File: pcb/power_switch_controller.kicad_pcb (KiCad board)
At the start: 2 copper layers, 118.1 x 54.6 mm, 63 parts, among them P1 PWR_JACK_2.5x5.5, P2 HEADER_01X03, P3 BNC_DOUBLE_RA, P4 HEADER_02X08_SMD, P5 HEADER_02X08_SMD, P6 HEADER_02X08_SMD, P7 HEADER_02X08_SMD, SW1 DPST_SERIES_M, SW2 KT_SWITCH, U1 MAX6817, U2 MAX6817, U3 TLE723X, U4 TLE723X, U5 TLE723X, U6 TLE723X

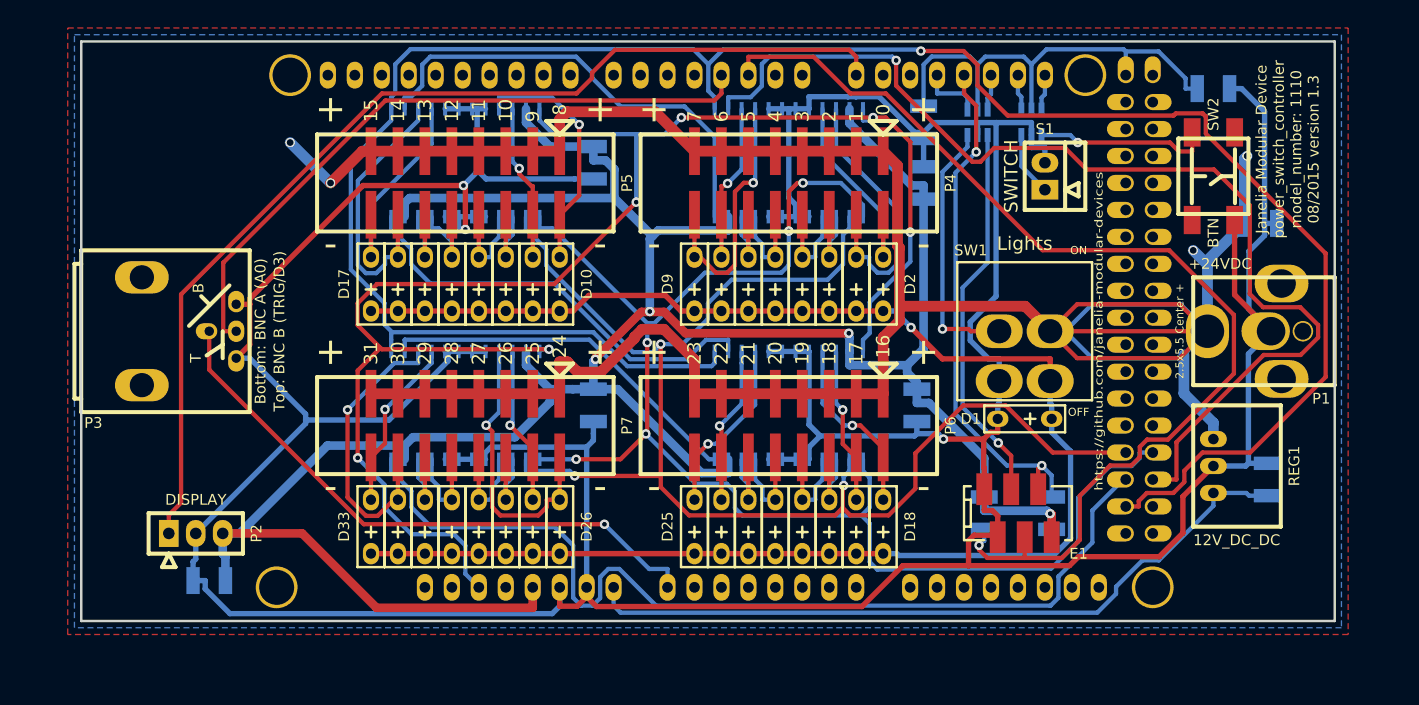
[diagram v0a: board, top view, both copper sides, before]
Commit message: Progress towards pcb v1.4.
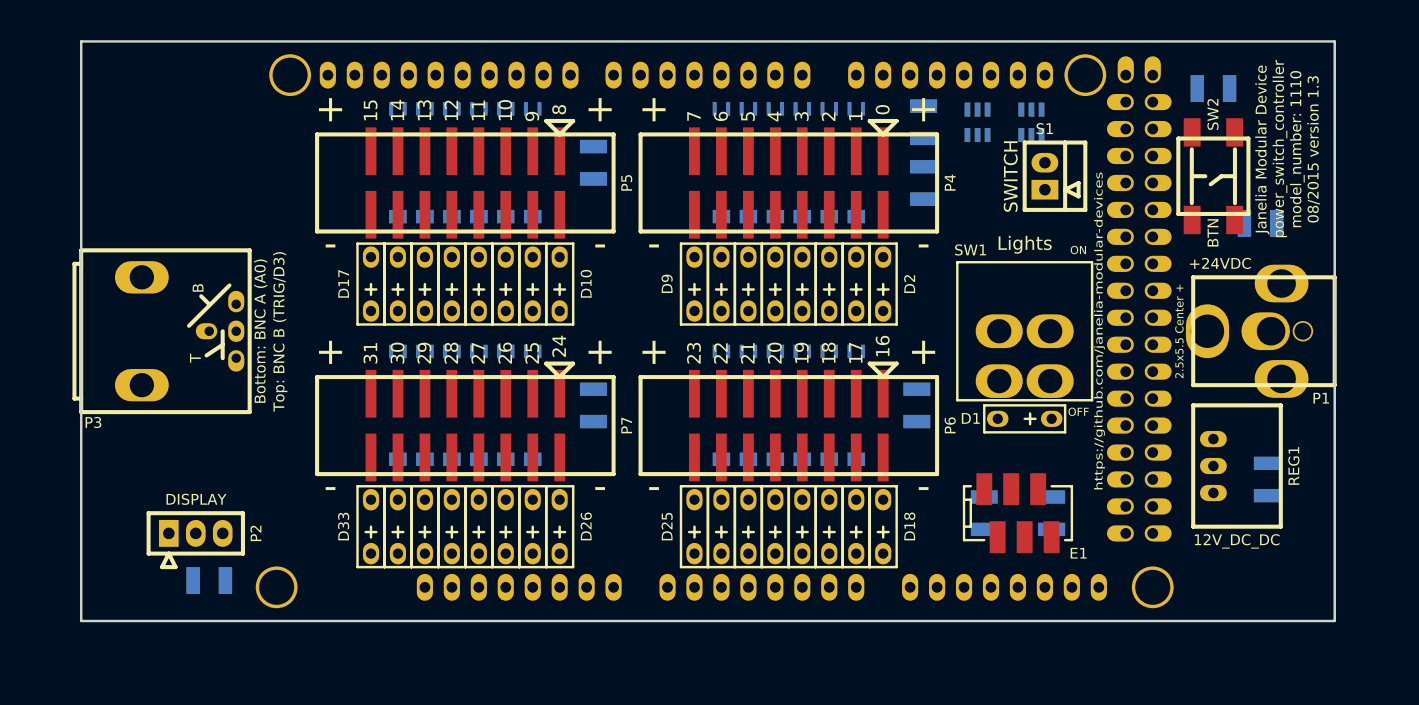
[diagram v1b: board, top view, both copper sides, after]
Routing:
- net GND: track 449.0 -> 0.00 mm, vias 3 -> 0
- net VAA: track 270.6 -> 0.00 mm, vias 4 -> 0
- net +5V: track 254.0 -> 0.00 mm, vias 4 -> 0
- net /SCK: track 203.9 -> 0.00 mm, vias 1 -> 0
- net /LED_PWR: track 151.6 -> 0.00 mm, vias 1 -> 0
- net /RST: track 151.1 -> 0.00 mm, vias 6 -> 0
- net /CS: track 137.5 -> 0.00 mm, vias 5 -> 0
- net /IN: track 131.6 -> 0.00 mm, vias 3 -> 0
- net /ENC_B: track 101.7 -> 0.00 mm, vias 1 -> 0
- net /MOSI: track 101.7 -> 0.00 mm, vias 1 -> 0
- net /TX3: track 98.5 -> 0.00 mm
- net /MISO: track 91.2 -> 0.00 mm
- net /V_IN: track 69.5 -> 0.00 mm
- net /BNC_B: track 63.0 -> 0.00 mm
- net /BNC_A: track 56.3 -> 0.00 mm, vias 1 -> 0
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- removed copper zone on B.Cu, net GND
- removed copper zone on F.Cu, net VAA

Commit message: Updated bom.
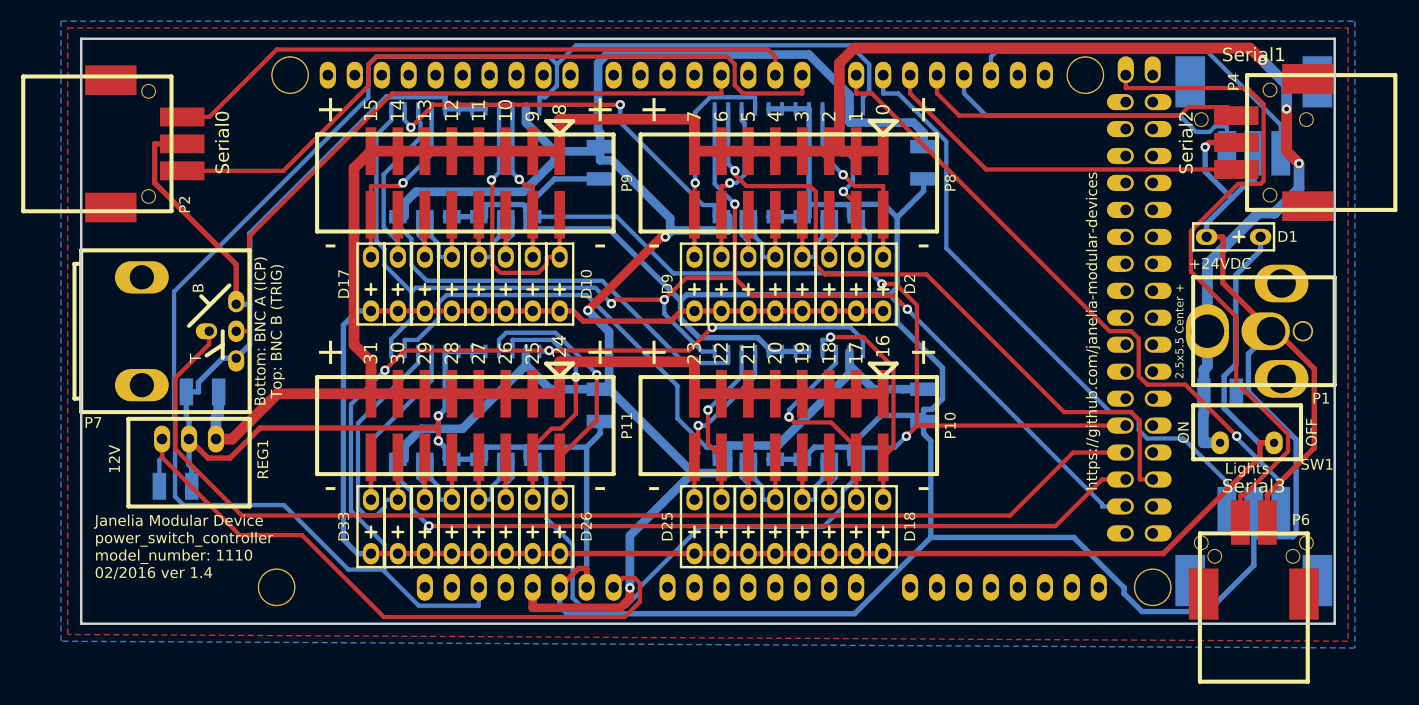
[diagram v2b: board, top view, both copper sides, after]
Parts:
- removed C8, C9: 0.1uF, power_switch_controller:SM1210
- removed E1: ENCODER_C14, power_switch_controller:Micro-MaTch_6_SMD
- removed R1, R2: 5.11k, power_switch_controller:SM1210
- removed S1: HEADER_01X02_SHR, power_switch_controller:Header_Shrouded_2_Pin
- removed SW2: KT_SWITCH, power_switch_controller:KT_SWITCH
- removed U5, U6: TLE723X, power_switch_controller:TLE723X
- added P10: HEADER_02X08_SMD, power_switch_controller:HEADER_02x08_SMD, F.Cu at (160.0, 111.8)
- added P11: HEADER_02X08_SMD, power_switch_controller:HEADER_02x08_SMD, F.Cu at (129.5, 111.8)
- added P8: HEADER_02X08_SMD, power_switch_controller:HEADER_02x08_SMD, F.Cu at (160.0, 88.9)
- added P9: HEADER_02X08_SMD, power_switch_controller:HEADER_02x08_SMD, F.Cu at (129.5, 88.9)
- P2: value HEADER_01X03 -> HEADER_01X03_SMD_RA; footprint footprints:Header_3_Pin -> power_switch_controller:Header_3_Pin_SMD_RA
- P3: value BNC_DOUBLE_RA -> HEADER_01X03_SMD_RA; footprint power_switch_controller:BNC_DOUBLE -> power_switch_controller:Header_3_Pin_SMD_RA; moved to B.Cu
- P4: value HEADER_02X08_SMD -> HEADER_01X03_SMD_RA; footprint power_switch_controller:HEADER_02x08_SMD -> power_switch_controller:Header_3_Pin_SMD_RA
- P5: value HEADER_02X08_SMD -> HEADER_01X03_SMD_RA; footprint power_switch_controller:HEADER_02x08_SMD -> power_switch_controller:Header_3_Pin_SMD_RA; moved to B.Cu
- P6: value HEADER_02X08_SMD -> HEADER_01X02_SMD_RA; footprint power_switch_controller:HEADER_02x08_SMD -> power_switch_controller:Header_2_Pin_SMD_RA
- P7: value HEADER_02X08_SMD -> BNC_DOUBLE_RA; footprint power_switch_controller:HEADER_02x08_SMD -> power_switch_controller:BNC_DOUBLE
- SW1: value DPST_SERIES_M -> SPST_SLIDE_AS; footprint power_switch_controller:DPST_SERIES_M -> power_switch_controller:SPST_SLIDE_AS
- U1, U2: value MAX6817 -> TLE723X; footprint power_switch_controller:MAX6817 -> power_switch_controller:TLE723X
- moved P3 107.4 mm to (203.8, 79.4), turned to 180 degrees
- moved C2 100.7 mm to (104.8, 108.6), turned to 180 degrees
- moved REG1 96.6 mm to (103.5, 113.0), turned to 180 degrees
- moved P5 83.2 mm to (203.8, 126.4)
- moved C5 58.2 mm to (142.2, 87.0), turned to 270 degrees
- moved U2 53.5 mm to (129.5, 87.0), turned to 180 degrees
- moved P4 49.0 mm to (208.9, 85.1), turned to 270 degrees
- moved P6 46.6 mm to (203.8, 127.6), turned to 180 degrees
- moved P2 37.6 mm to (96.1, 85.2), turned to 90 degrees
- moved P7 31.7 mm to (99.1, 102.9), turned to 90 degrees
- moved D1 26.1 mm to (201.9, 94.0)
- moved SW1 23.0 mm to (203.2, 112.4), turned to 90 degrees
- moved C7 22.9 mm to (142.2, 109.9)
- moved U3 22.9 mm to (160.0, 109.9)
- moved U4 22.9 mm to (129.5, 109.9)
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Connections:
- ARDUINO1 pad 0: Net-(ARDUINO1-Pad0) -> /RX0
- ARDUINO1 pad 1: Net-(ARDUINO1-Pad1) -> /TX0
- ARDUINO1 pad 10: Net-(ARDUINO1-Pad10) -> (no net)
- ARDUINO1 pad 11: Net-(ARDUINO1-Pad11) -> (no net)
- ARDUINO1 pad 12: Net-(ARDUINO1-Pad12) -> (no net)
- ARDUINO1 pad 13: Net-(ARDUINO1-Pad13) -> (no net)
- ARDUINO1 pad 15: Net-(ARDUINO1-Pad15) -> /RX3
- ARDUINO1 pad 16: Net-(ARDUINO1-Pad16) -> /TX2
- ARDUINO1 pad 17: /D_LIGHTS -> /RX2
- ARDUINO1 pad 18: /ENC_A -> /TX1
- ARDUINO1 pad 19: /D_ENC_BTN -> /RX1
- ARDUINO1 pad 2: /ENC_B -> (no net)
- ARDUINO1 pad 20: /D_SWITCH -> (no net)
- ARDUINO1 pad 20B: Net-(ARDUINO1-Pad20B) -> (no net)
- ARDUINO1 pad 21: /D_BTN -> (no net)
- ARDUINO1 pad 21B: Net-(ARDUINO1-Pad21B) -> (no net)
- ARDUINO1 pad 22: Net-(ARDUINO1-Pad22) -> (no net)
- ARDUINO1 pad 23: Net-(ARDUINO1-Pad23) -> (no net)
- ARDUINO1 pad 24: Net-(ARDUINO1-Pad24) -> (no net)
- ARDUINO1 pad 25: Net-(ARDUINO1-Pad25) -> (no net)
- ARDUINO1 pad 26: Net-(ARDUINO1-Pad26) -> (no net)
- ARDUINO1 pad 27: Net-(ARDUINO1-Pad27) -> (no net)
- ARDUINO1 pad 28: Net-(ARDUINO1-Pad28) -> (no net)
- ARDUINO1 pad 29: Net-(ARDUINO1-Pad29) -> (no net)
- ARDUINO1 pad 30: Net-(ARDUINO1-Pad30) -> (no net)
- ARDUINO1 pad 31: Net-(ARDUINO1-Pad31) -> (no net)
- ARDUINO1 pad 32: Net-(ARDUINO1-Pad32) -> (no net)
- ARDUINO1 pad 33: Net-(ARDUINO1-Pad33) -> (no net)
- ARDUINO1 pad 34: Net-(ARDUINO1-Pad34) -> (no net)
- ARDUINO1 pad 35: Net-(ARDUINO1-Pad35) -> (no net)
- ARDUINO1 pad 36: Net-(ARDUINO1-Pad36) -> (no net)
- ARDUINO1 pad 37: Net-(ARDUINO1-Pad37) -> (no net)
- ARDUINO1 pad 38: Net-(ARDUINO1-Pad38) -> (no net)
- ARDUINO1 pad 39: Net-(ARDUINO1-Pad39) -> (no net)
- ARDUINO1 pad 3V3: Net-(ARDUINO1-Pad3V3) -> (no net)
- ARDUINO1 pad 4: Net-(ARDUINO1-Pad4) -> (no net)
- ARDUINO1 pad 40: Net-(ARDUINO1-Pad40) -> (no net)
- ARDUINO1 pad 41: Net-(ARDUINO1-Pad41) -> (no net)
- ARDUINO1 pad 42: Net-(ARDUINO1-Pad42) -> (no net)
- ARDUINO1 pad 43: Net-(ARDUINO1-Pad43) -> (no net)
- ARDUINO1 pad 44: Net-(ARDUINO1-Pad44) -> (no net)
- ARDUINO1 pad 45: Net-(ARDUINO1-Pad45) -> (no net)
- ARDUINO1 pad 46: Net-(ARDUINO1-Pad46) -> /CS
- ARDUINO1 pad 47: Net-(ARDUINO1-Pad47) -> (no net)
- ARDUINO1 pad 48: /IN -> /BNC_A
- ARDUINO1 pad 49: /CS -> (no net)
- ARDUINO1 pad 5: Net-(ARDUINO1-Pad5) -> (no net)
- ARDUINO1 pad 53: Net-(ARDUINO1-Pad53) -> (no net)
- ARDUINO1 pad 5V_5: Net-(ARDUINO1-Pad5V_5) -> (no net)
- ARDUINO1 pad 6: Net-(ARDUINO1-Pad6) -> (no net)
- ARDUINO1 pad 7: Net-(ARDUINO1-Pad7) -> (no net)
- ARDUINO1 pad 8: Net-(ARDUINO1-Pad8) -> (no net)
- ARDUINO1 pad 9: Net-(ARDUINO1-Pad9) -> (no net)
- ARDUINO1 pad A0: /BNC_A -> (no net)
- ARDUINO1 pad A1: Net-(ARDUINO1-PadA1) -> (no net)
- ARDUINO1 pad A10: Net-(ARDUINO1-PadA10) -> (no net)
- ARDUINO1 pad A11: Net-(ARDUINO1-PadA11) -> (no net)
- ARDUINO1 pad A12: Net-(ARDUINO1-PadA12) -> (no net)
- ARDUINO1 pad A13: Net-(ARDUINO1-PadA13) -> (no net)
- ARDUINO1 pad A14: Net-(ARDUINO1-PadA14) -> (no net)
- ARDUINO1 pad A15: Net-(ARDUINO1-PadA15) -> (no net)
- ARDUINO1 pad A2: Net-(ARDUINO1-PadA2) -> (no net)
- ARDUINO1 pad A3: Net-(ARDUINO1-PadA3) -> (no net)
- ARDUINO1 pad A4: Net-(ARDUINO1-PadA4) -> (no net)
- ARDUINO1 pad A5: Net-(ARDUINO1-PadA5) -> (no net)
- ARDUINO1 pad A6: Net-(ARDUINO1-PadA6) -> (no net)
- ARDUINO1 pad A7: Net-(ARDUINO1-PadA7) -> (no net)
- ARDUINO1 pad A8: Net-(ARDUINO1-PadA8) -> (no net)
- ARDUINO1 pad A9: Net-(ARDUINO1-PadA9) -> (no net)
- ARDUINO1 pad AREF: Net-(ARDUINO1-PadAREF) -> (no net)
- ARDUINO1 pad GND3: Net-(ARDUINO1-PadGND3) -> (no net)
- ARDUINO1 pad GND4: Net-(ARDUINO1-PadGND4) -> (no net)
- ARDUINO1 pad GND5: Net-(ARDUINO1-PadGND5) -> (no net)
- ARDUINO1 pad IREF: Net-(ARDUINO1-PadIREF) -> (no net)
- ARDUINO1 pad NC: Net-(ARDUINO1-PadNC) -> (no net)
- C2 pad 1: /V_IN -> VAA
- C3 pad 1: +5V -> /V_IN
- C4 pad 1: +5VD -> +5V
- C5 pad 1: +5VD -> +5V
- P2 pad 1: /TX3 -> /RX0
- P2 pad 3: +5V -> /TX0
- P3 pad 1: /BNC_A -> /RX1
- P3 pad 3: /BNC_B -> /TX1
- P4 pad 1: VAA -> /RX2
- P4 pad 2: /OUT0 -> GND
- P4 pad 3: VAA -> /TX2
- P5 pad 1: VAA -> /RX3
- P5 pad 2: /OUT8 -> GND
- P5 pad 3: VAA -> /TX3
- P6 pad 1: VAA -> GND
- P6 pad 2: /OUT16 -> +5VD
- P7 pad 1: VAA -> /BNC_A
- P7 pad 2: /OUT24 -> GND
- P7 pad 3: VAA -> /BNC_B
- P7 pad 4: /OUT25 -> GND
- U1 pad 1: /ENC_BTN -> /CS
- U1 pad 3: /LIGHTS -> /OUT2
- U1 pad 4: /D_LIGHTS -> /OUT3
- U1 pad 5: +5VD -> GND
- U1 pad 6: /D_ENC_BTN -> GND
- U2 pad 1: /BTN -> /CS
- U2 pad 3: /SWITCH -> /OUT10
- U2 pad 4: /D_SWITCH -> /OUT11
- U2 pad 5: +5VD -> GND
- U2 pad 6: /D_BTN -> GND
- U3 pad 10: /OUT5 -> /OUT21
- U3 pad 12: /SI1 -> /SI3
- U3 pad 14: /MOSI -> /SI2
- U3 pad 15: /OUT6 -> /OUT22
- U3 pad 16: /OUT7 -> /OUT23
- U3 pad 2: /IN -> GND
- U3 pad 21: /OUT0 -> /OUT16
- U3 pad 22: /OUT1 -> /OUT17
- U3 pad 3: /OUT2 -> /OUT18
- U3 pad 4: /OUT3 -> /OUT19
- U3 pad 9: /OUT4 -> /OUT20
- U4 pad 10: /OUT13 -> /OUT29
- U4 pad 12: /SI2 -> /MISO
- U4 pad 14: /SI1 -> /SI3
- U4 pad 15: /OUT14 -> /OUT30
- U4 pad 16: /OUT15 -> /OUT31
- U4 pad 2: /IN -> GND
- U4 pad 21: /OUT8 -> /OUT24
- U4 pad 22: /OUT9 -> /OUT25
- U4 pad 3: /OUT10 -> /OUT26
- U4 pad 4: /OUT11 -> /OUT27
- U4 pad 9: /OUT12 -> /OUT28
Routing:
- net GND: track 0.00 -> 472.6 mm, vias 0 -> 3
- net VAA: track 0.00 -> 246.7 mm, vias 0 -> 3
- net /RST: track 0.00 -> 212.6 mm, vias 0 -> 3
- net +5V: track 0.00 -> 202.4 mm, vias 0 -> 3
- net /LED_PWR: track 0.00 -> 189.4 mm
- net /CS: track 0.00 -> 132.3 mm, vias 0 -> 2
- net /SCK: track 0.00 -> 128.0 mm, vias 0 -> 4
- net /BNC_A: track 0.00 -> 107.0 mm
- net /MISO: track 0.00 -> 75.2 mm, vias 0 -> 1
- net /RX0: track 0.00 -> 68.4 mm
- net /MOSI: track 0.00 -> 65.0 mm, vias 0 -> 1
- net +5VD: track 0.00 -> 64.2 mm
- net /V_IN: track 0.00 -> 62.9 mm
- net /BNC_B: track 0.00 -> 61.9 mm
- net /TX3: track 0.00 -> 61.6 mm, vias 0 -> 1
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- added copper zone on B.Cu, net GND
- added copper zone on F.Cu, net VAA
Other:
- board size 118.1 x 54.6 mm -> 118.1 x 55.1 mm
- board text added: "12V"
- board text added: "Janelia Modular Device power_switch_controller model_number: 1110 02/2016 ver 1.4"
- board text added: "Lights"
- board text added: "Serial0"
- board text added: "Serial1"
- board text added: "Serial2"
- board text added: "Serial3"
- board text removed: "12V_DC_DC"
- board text removed: "DISPLAY"
- board text removed: "Janelia Modular Device power_switch_controller model_number: 1110 08/2015 version 1.3"
- board text removed: "SWITCH"
